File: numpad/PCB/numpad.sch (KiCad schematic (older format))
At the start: 46 parts

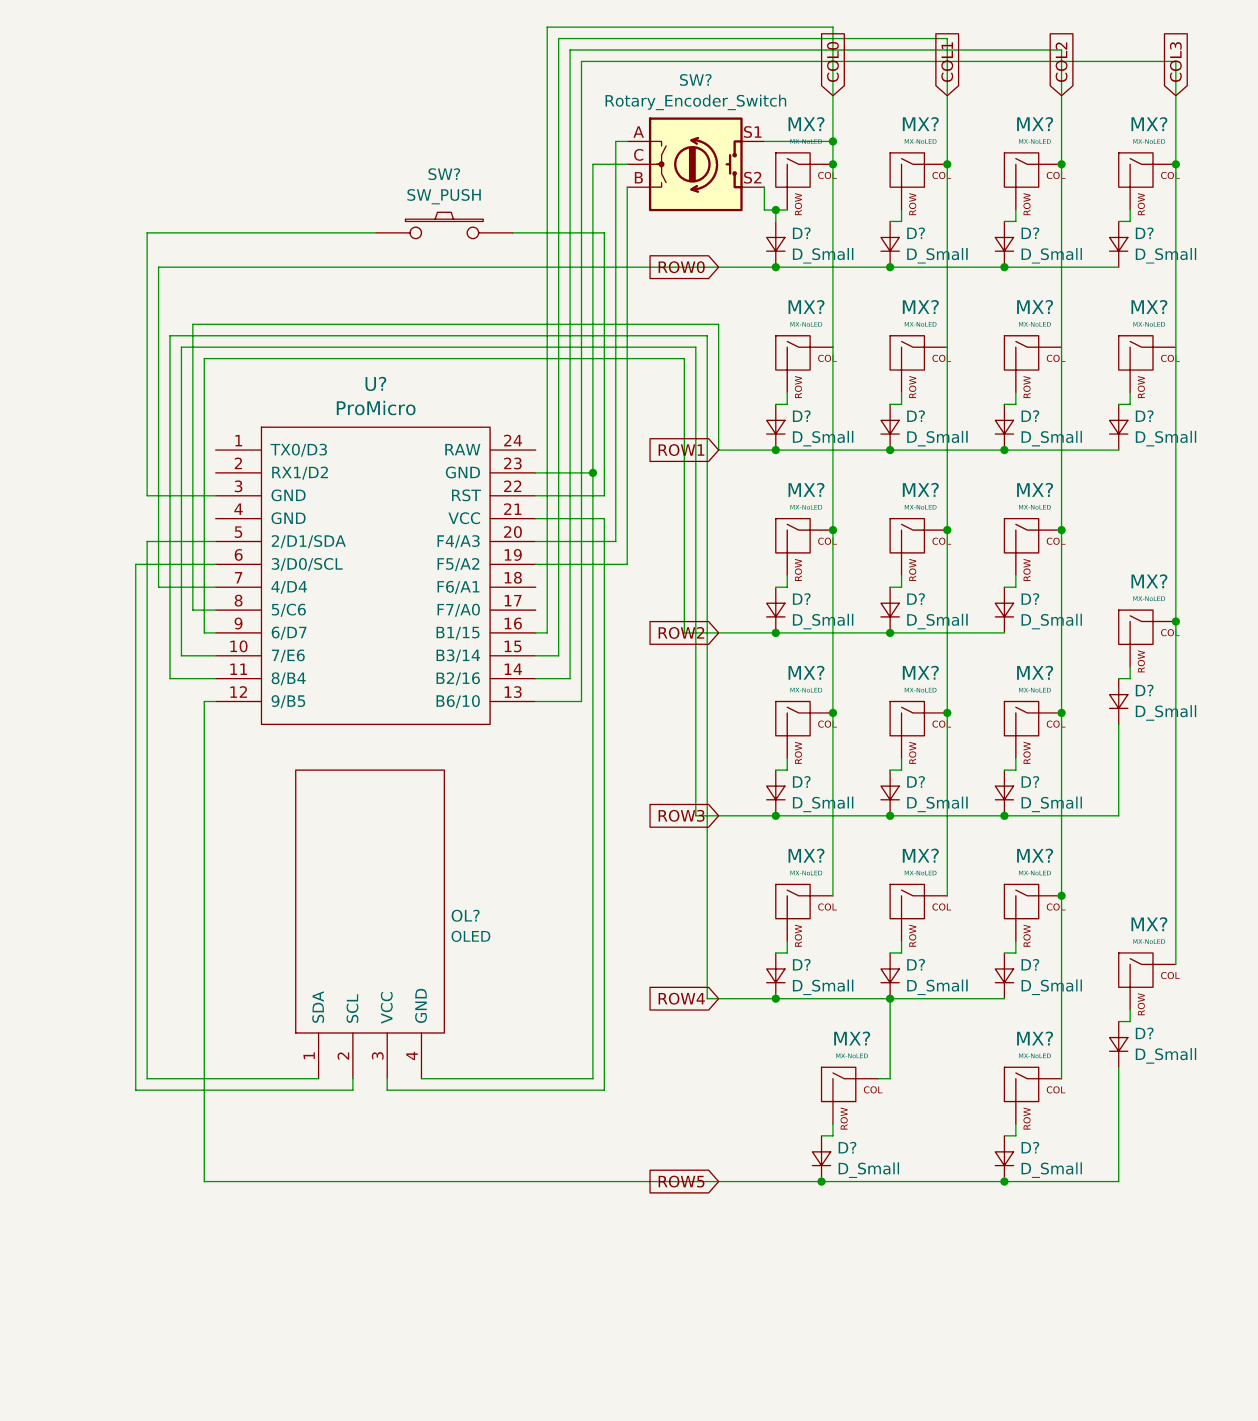
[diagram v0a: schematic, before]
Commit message: Pretty much made the entire thing this commit
Auto routed kek
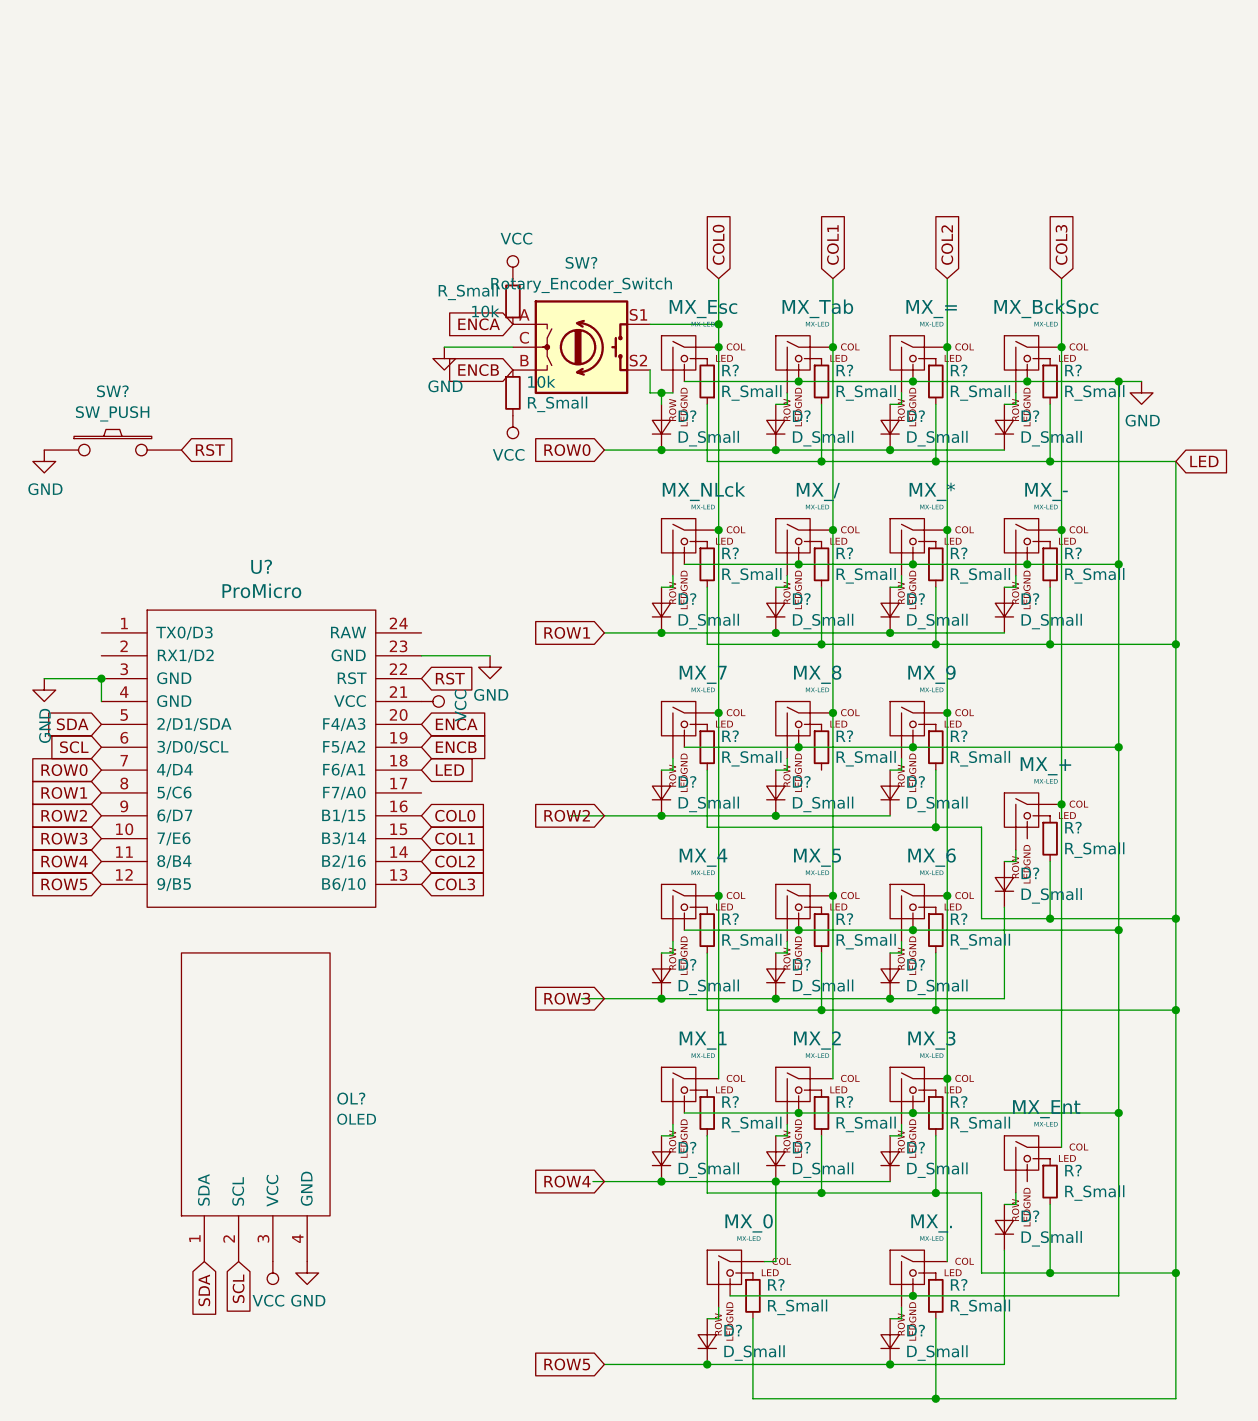
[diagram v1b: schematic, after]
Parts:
- removed MX? (x21): MX-NoLED, symbol MX_Alps_Hybrid:MX-NoLED
- added 10k (x2), R? (x21): R_Small, symbol Device:R_Small
- added MX_*, MX_+, MX_-, MX_., MX_/, MX_0, MX_1, MX_2, MX_3, MX_4, MX_5, MX_6, MX_7, MX_8, MX_9, MX_=, MX_BckSpc, MX_Ent, MX_Esc, MX_NLck, MX_Tab: MX-LED, symbol MX_Alps_Hybrid:MX-LED
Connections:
- net COL0: now also MX_1.1 (COL), MX_4.1 (COL), MX_7.1 (COL), MX_Esc.1 (COL), MX_NLck.1 (COL)
- net COL1: now also MX_/.1 (COL), MX_2.1 (COL), MX_5.1 (COL), MX_8.1 (COL), MX_Tab.1 (COL)
- net COL2: now also MX_*.1 (COL), MX_..1 (COL), MX_3.1 (COL), MX_6.1 (COL), MX_9.1 (COL), MX_=.1 (COL)
- net COL3: now also MX_+.1 (COL), MX_-.1 (COL), MX_BckSpc.1 (COL), MX_Ent.1 (COL)
- net ROW4: now also MX_0.1 (COL)
- net at D?.2 (A): now also MX_7.2 (ROW)
- net at D?.2 (A): now also MX_8.2 (ROW)
- net at D?.2 (A): now also MX_9.2 (ROW)
- net at D?.2 (A): now also MX_+.2 (ROW)
- net ENCA: now reaches SW?.A, U?.20 (F4/A3)
- net ENCA: now also 10k.1
- net ENCB: now reaches SW?.B, U?.19 (F5/A2)
- net ENCB: now also 10k.1
- net GND: now reaches OL?.4 (GND), SW?.C, U?.23 (GND)
- net GND: now also SW?.1, U?.3 (GND), U?.4 (GND), MX_*.4 (LEDGND), MX_-.4 (LEDGND), MX_..4 (LEDGND), MX_/.4 (LEDGND), MX_0.4 (LEDGND), MX_1.4 (LEDGND), MX_2.4 (LEDGND), MX_3.4 (LEDGND), MX_4.4 (LEDGND), MX_5.4 (LEDGND), MX_6.4 (LEDGND), MX_7.4 (LEDGND), MX_8.4 (LEDGND), MX_9.4 (LEDGND), MX_=.4 (LEDGND), MX_BckSpc.4 (LEDGND), MX_Esc.4 (LEDGND), MX_NLck.4 (LEDGND), MX_Tab.4 (LEDGND)
- net at D?.2 (A), SW?.S2: now also MX_Esc.2 (ROW)
- net at D?.2 (A): now also MX_4.2 (ROW)
- net at D?.2 (A): now also MX_5.2 (ROW)
- net at D?.2 (A): now also MX_6.2 (ROW)
- net at D?.2 (A): now also MX_Ent.2 (ROW)
- net at D?.2 (A): now also MX_1.2 (ROW)
- net at D?.2 (A): now also MX_2.2 (ROW)
- net at D?.2 (A): now also MX_3.2 (ROW)
- net at D?.2 (A): now also MX_0.2 (ROW)
- net at D?.2 (A): now also MX_..2 (ROW)
- net at D?.2 (A): now also MX_NLck.2 (ROW)
- net at D?.2 (A): now also MX_/.2 (ROW)
- net at D?.2 (A): now also MX_*.2 (ROW)
- net at D?.2 (A): now also MX_-.2 (ROW)
- net at D?.2 (A): now also MX_Tab.2 (ROW)
- net at D?.2 (A): now also MX_=.2 (ROW)
- net at D?.2 (A): now also MX_BckSpc.2 (ROW)
- net LED: now reaches U?.18 (F6/A1)
- net LED: now also R?.1, R?.2, R?.2, R?.2, R?.2, R?.2, R?.2, R?.2, R?.2, R?.2, R?.2, R?.2, R?.2, R?.2, R?.2, R?.2, R?.2, R?.2, R?.2, R?.2
- net VCC: now reaches OL?.3 (VCC), U?.21 (VCC)
- net VCC: now also 10k.2, 10k.2
- net RST: now reaches SW?.2, U?.22 (RST)
- net SDA: now reaches OL?.1 (SDA), U?.5 (2/D1/SDA)
- net SCL: now reaches OL?.2 (SCL), U?.6 (3/D0/SCL)
- new net: MX_Esc.3 (LED), R?.2
- new net: MX_Tab.3 (LED), R?.1
- new net: MX_=.3 (LED), R?.1
- new net: MX_BckSpc.3 (LED), R?.1
- new net: MX_NLck.3 (LED), R?.1
- new net: MX_/.3 (LED), R?.1
- new net: MX_*.3 (LED), R?.1
- new net: MX_-.3 (LED), R?.1
- new net: MX_7.3 (LED), R?.1
- new net: MX_8.3 (LED), R?.1
- new net: MX_9.3 (LED), R?.1
- new net: MX_+.3 (LED), R?.1
- new net: MX_4.3 (LED), R?.1
- new net: MX_5.3 (LED), R?.1
- new net: MX_6.3 (LED), R?.1
- new net: MX_1.3 (LED), R?.1
- new net: MX_2.3 (LED), R?.1
- new net: MX_3.3 (LED), R?.1
- new net: MX_Ent.3 (LED), R?.1
- new net: MX_..3 (LED), R?.1
- new net: MX_0.3 (LED), R?.1
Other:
- moved on the sheet: D?, OL?, SW?, U?
